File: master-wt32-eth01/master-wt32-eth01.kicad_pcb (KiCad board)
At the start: 2 copper layers, 69.9 x 72.4 mm, 23 parts, among them J1 24V Field, J2 24V System, J3 Enable, J4 Screw_Terminal_01x03, J5 Conn_01x06_Female, J6 Conn_01x06_Female, SW1 SW_DIP_x03, U1 LM2596-Board, U2 WT32-ETH0-Board, U3 PC817

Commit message: upgrade master-wt32-eth01 format
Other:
- net class Default removed
- net class Power removed

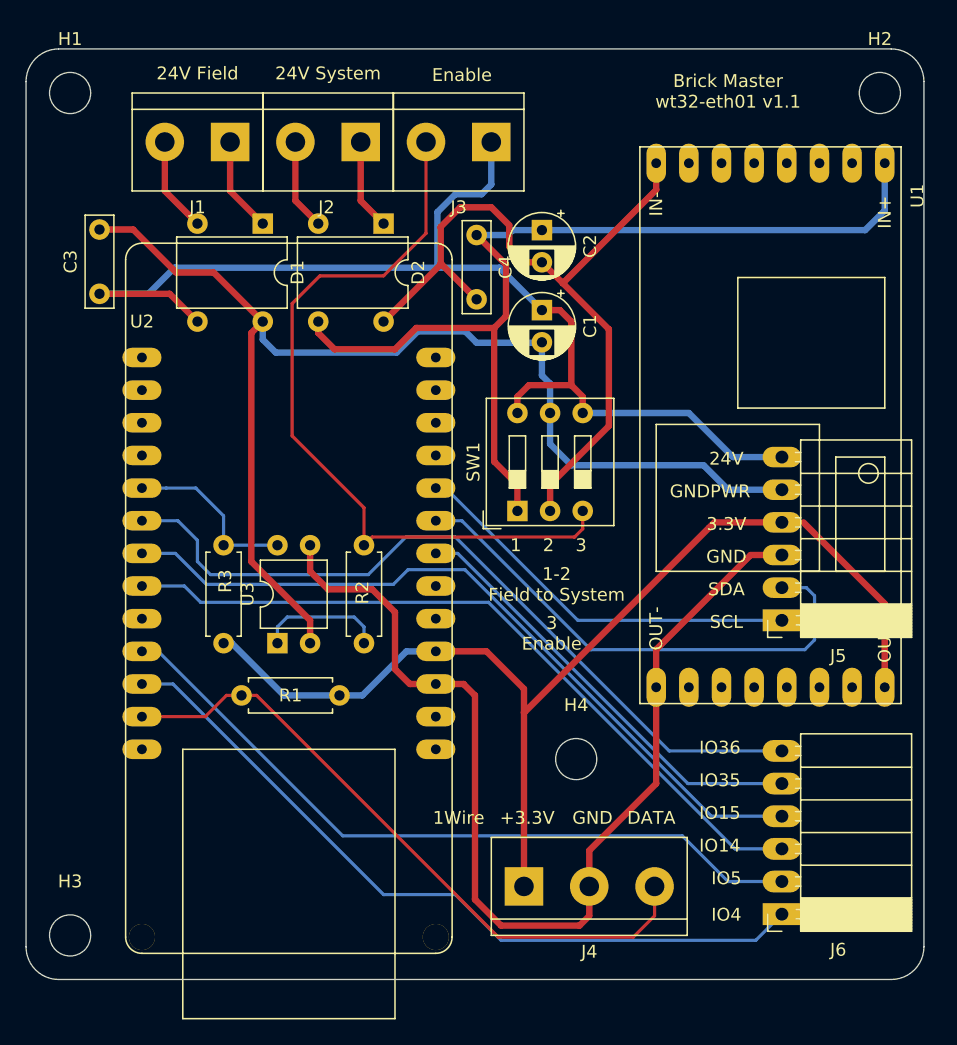
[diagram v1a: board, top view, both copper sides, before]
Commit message: refactor power
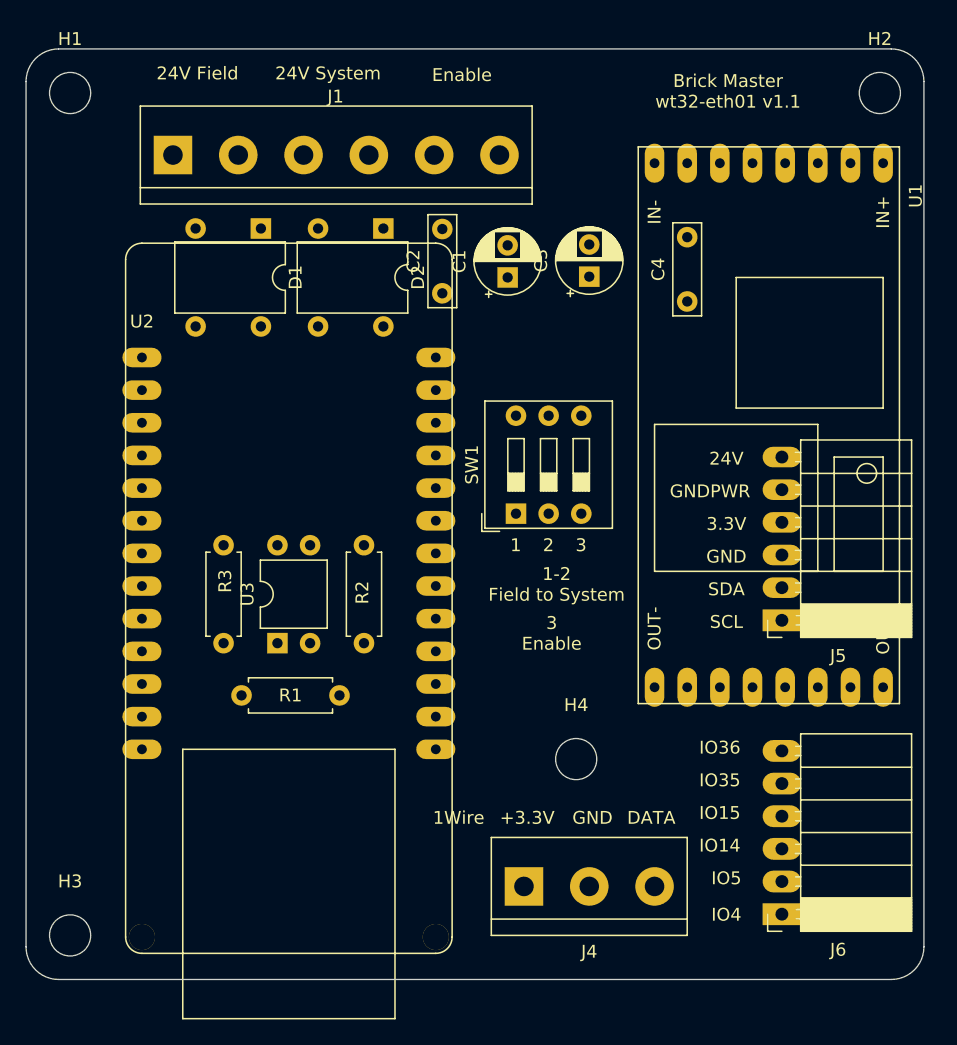
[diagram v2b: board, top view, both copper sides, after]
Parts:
- removed J2: 24V System, TerminalBlock:TerminalBlock_bornier-2_P5.08mm
- removed J3: Enable, TerminalBlock:TerminalBlock_bornier-2_P5.08mm
- C2: value 1uF 50V -> 100nF 50V; footprint Capacitor_THT:CP_Radial_D5.0mm_P2.50mm -> Capacitor_THT:C_Rect_L7.0mm_W2.0mm_P5.00mm
- C3: value 100nF 63V -> 1uF 50V; footprint Capacitor_THT:C_Rect_L7.0mm_W2.0mm_P5.00mm -> Capacitor_THT:CP_Radial_D5.0mm_P2.50mm
- J1: value 24V Field -> Screw_Terminal_01x06; footprint TerminalBlock:TerminalBlock_bornier-2_P5.08mm -> TerminalBlock:TerminalBlock_bornier-6_P5.08mm
- moved C3 38.1 mm to (107.3, 72.3)
- moved C4 17.2 mm to (114.9, 74.3), turned to 90 degrees
- moved C2 9.17 mm to (95.9, 73.6), turned to 90 degrees
- moved J1 4.56 mm to (74.9, 62.9), turned to 0 degrees
- moved C1 3.68 mm to (101.0, 72.4), turned to 90 degrees
- moved D1 0.41 mm to (81.8, 68.6)
- moved D2 0.38 mm to (91.3, 68.6)
- moved SW1 0.24 mm to (101.6, 90.8)
- moved U1 0.13 mm to (121.3, 83.8)
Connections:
- C2 pad 1: SYSTEM+ -> +24V
- C2 pad 2: SYSTEM- -> GNDPWR
- C3 pad 1: +24V -> +3V3
- C3 pad 2: GNDPWR -> GND
- C4 pad 1: SYSTEM+ -> +3V3
- C4 pad 2: SYSTEM- -> GND
- D1 pad 1: FIELD_IN- -> FIELD-
- D1 pad 2: FIELD_IN+ -> FIELD+
- D2 pad 1: SYSTEM_IN- -> SYSTEM-
- D2 pad 2: SYSTEM_IN+ -> SYSTEM+
- D2 pad 3: SYSTEM+ -> Net-(D2-Pad3)
- D2 pad 4: SYSTEM- -> Net-(D2-Pad4)
- J1 pad 1: FIELD_IN- -> FIELD+
- J1 pad 2: FIELD_IN+ -> FIELD-
- R2 pad 2: Net-(J3-Pad2) -> ENABLE_IN
- SW1 pad 1: SYSTEM+ -> FIELD+
- SW1 pad 2: SYSTEM- -> FIELD-
- SW1 pad 3: Net-(J3-Pad2) -> +24V
- SW1 pad 4: +24V -> ENABLE_IN
- SW1 pad 5: GNDPWR -> SYSTEM+
- SW1 pad 6: +24V -> SYSTEM+
- U1 pad 1: SYSTEM+ -> Net-(D2-Pad3)
- U1 pad 2: SYSTEM- -> Net-(D2-Pad4)
- U2 pad 1: Net-(U2-Pad1) -> unconnected-(U2-Pad1)
- U2 pad 12: Net-(U2-Pad12) -> unconnected-(U2-Pad12)
- U2 pad 13: Net-(U2-Pad13) -> unconnected-(U2-Pad13)
- U2 pad 14: Net-(U2-Pad14) -> unconnected-(U2-Pad14)
- U2 pad 18: Net-(U2-Pad18) -> unconnected-(U2-Pad18)
- U2 pad 2: Net-(U2-Pad2) -> unconnected-(U2-Pad2)
- U2 pad 23: Net-(U2-Pad23) -> unconnected-(U2-Pad23)
- U2 pad 24: Net-(U2-Pad24) -> unconnected-(U2-Pad24)
- U2 pad 25: Net-(U2-Pad25) -> unconnected-(U2-Pad25)
- U2 pad 26: Net-(U2-Pad26) -> unconnected-(U2-Pad26)
- U2 pad 3: Net-(U2-Pad3) -> unconnected-(U2-Pad3)
- U2 pad 4: Net-(U2-Pad4) -> unconnected-(U2-Pad4)
- U2 pad 8: Net-(U2-Pad8) -> unconnected-(U2-Pad8)
- U2 pad 9: Net-(U2-Pad9) -> unconnected-(U2-Pad9)
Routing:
- net GNDPWR: track 95.2 -> 0.00 mm
- net +24V: track 90.7 -> 0.00 mm
- net +3V3: track 84.7 -> 0.00 mm
- net GND: track 83.1 -> 0.00 mm
- net SYSTEM+: track 75.6 -> 0.00 mm
- net GPIO36: track 60.6 -> 0.00 mm
- net SYSTEM-: track 60.1 -> 0.00 mm
- net Net-(J3-Pad2): track 59.8 -> 0.00 mm
- net GPIO15: track 59.2 -> 0.00 mm
- net GPIO4: track 58.9 -> 0.00 mm
- net GPIO14: track 58.3 -> 0.00 mm
- net GPIO5: track 57.2 -> 0.00 mm
- net 1WIRE: track 51.3 -> 0.00 mm
- net SDA: track 40.2 -> 0.00 mm
- net GPIO35: track 34.3 -> 0.00 mm
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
